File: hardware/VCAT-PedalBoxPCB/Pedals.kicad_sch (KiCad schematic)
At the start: 18 parts, among them U3 TLV9301xDCK, U6 TLV9301xDCK

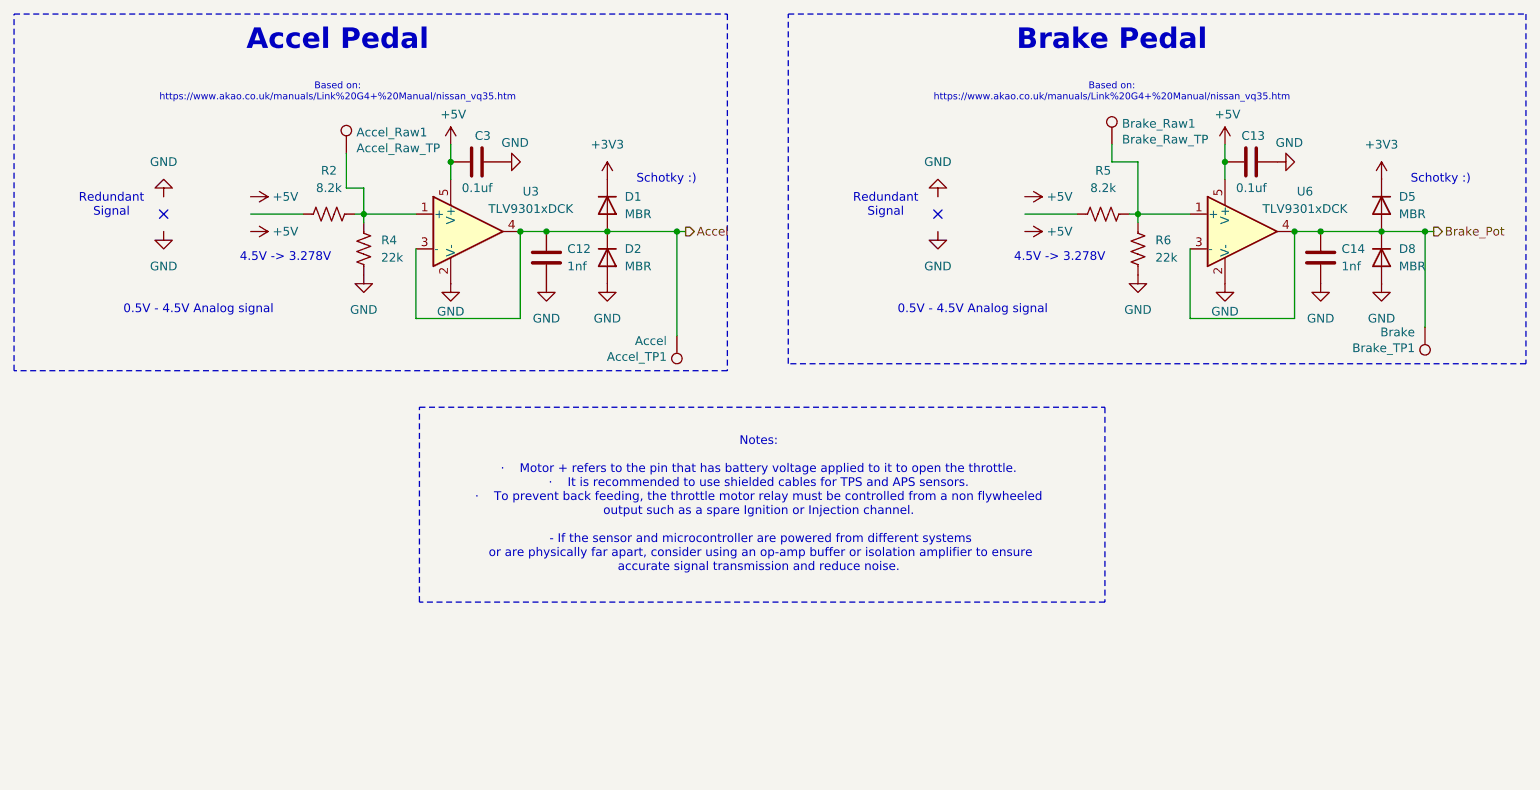
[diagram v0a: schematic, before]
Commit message: sch too ez
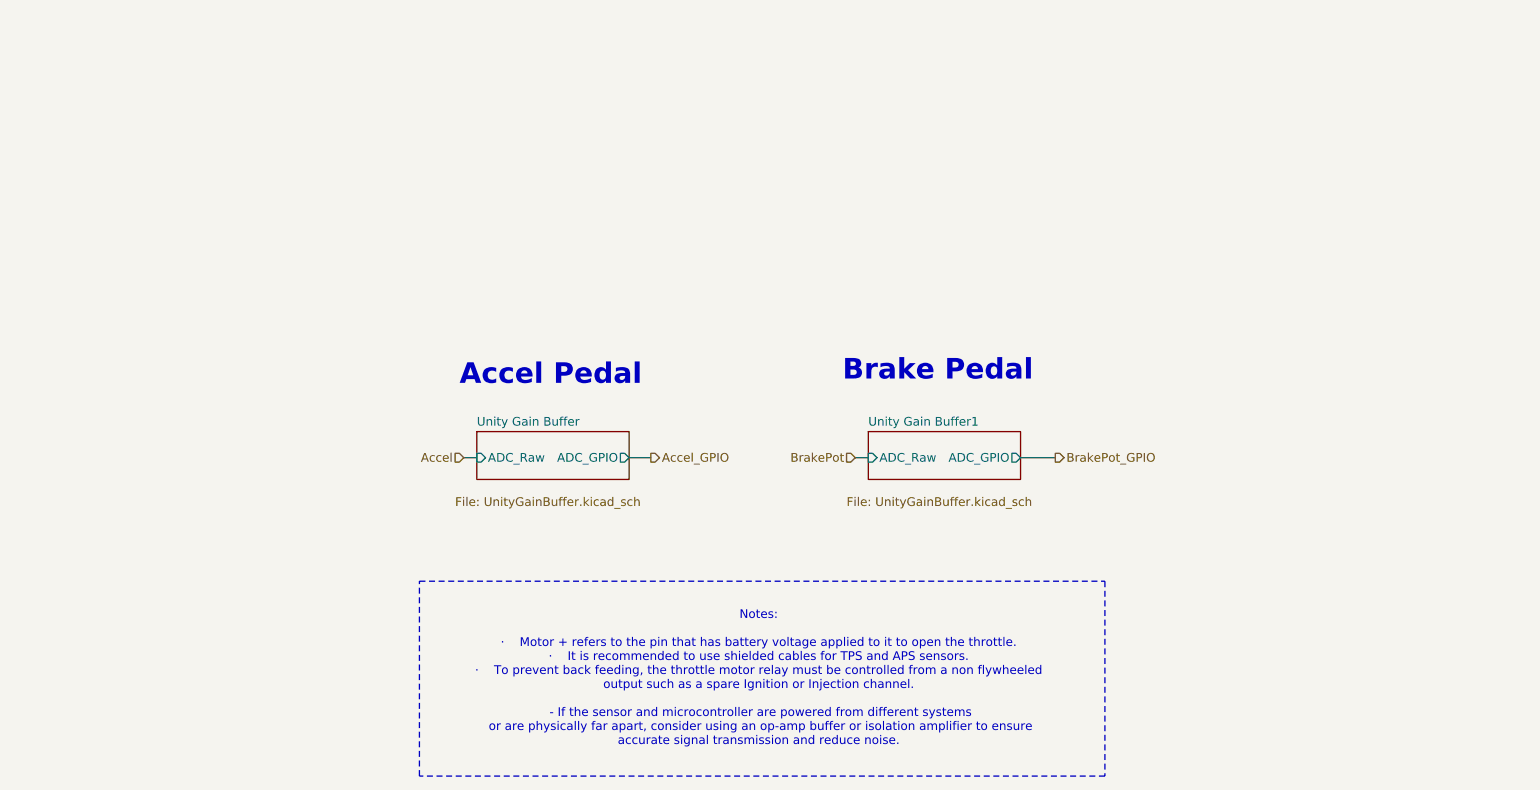
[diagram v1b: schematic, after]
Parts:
- removed Accel_Raw1: Accel_Raw_TP, TestPoint:TestPoint_THTPad_1.5x1.5mm_Drill0.7mm, symbol Connector:TestPoint
- removed Accel_TP1: Accel, TestPoint:TestPoint_THTPad_1.5x1.5mm_Drill0.7mm, symbol Connector:TestPoint
- removed Brake_Raw1: Brake_Raw_TP, TestPoint:TestPoint_THTPad_1.5x1.5mm_Drill0.7mm, symbol Connector:TestPoint
- removed Brake_TP1: Brake, TestPoint:TestPoint_THTPad_1.5x1.5mm_Drill0.7mm, symbol Connector:TestPoint
- removed C12, C14: 1nf, Capacitor_SMD:C_0805_2012Metric, symbol Device:C
- removed C13, C3: 0.1uf, Capacitor_SMD:C_0805_2012Metric, symbol Device:C
- removed D1, D2, D5, D8: MBR, Diode_SMD:D_0805_2012Metric, symbol Device:D
- removed R2, R5: 8.2k, Resistor_SMD:R_0805_2012Metric, symbol Device:R_US
- removed R4, R6: 22k, Resistor_SMD:R_0805_2012Metric, symbol Device:R_US
- removed U3, U6: TLV9301xDCK, Package_TO_SOT_SMD:SOT-353_SC-70-5, symbol Amplifier_Operational:TLV9301xDCK
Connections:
- no-connect marks 2 -> 0
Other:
- added sheet Unity Gain Buffer (UnityGainBuffer.kicad_sch)
- added sheet Unity Gain Buffer1 (UnityGainBuffer.kicad_sch)
- note removed: "0.5V - 4.5V Analog signal"
- note removed: "4.5V -> 3.278V"
- note removed: "Based on: https://www.akao.co.uk/manuals/Link%20G4+%20Manual/nissan_vq35.htm"
- note removed: "Redundant Signal"
- note removed: "Schotky :)"
